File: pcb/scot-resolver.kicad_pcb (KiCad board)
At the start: 2 copper layers, 108.5 x 79.2 mm, 148 parts, among them IC1 AD8692ARMZ, IC10 AD2S1210, IC2 AD8397ARZ, IC3 AD8692ARMZ, IC4 TSR1, IC5 AD8692ARMZ, IC6 AD8692ARMZ, IC7 AD8692ARMZ, IC8 MCP2562, IC9 STM32F0xxKxTx, J1 Conn_01x02_Female, J2 Conn_01x02_Female, J3 Conn_01x02_Female, J4 Conn_01x03_Female, J5 Conn_01x03_Female, J6 Conn_01x03_Female, J7 CONN_01x03, P1 SWD, U1 MCP1703A-5002_SOT223, U2 LT1762, U3 MCP1703A-5002_SOT223, U4 MCP1703A-5002_SOT223, U5 MCP1703A-3302_SOT223, Y1 Crystal_GND24, Y2 Crystal

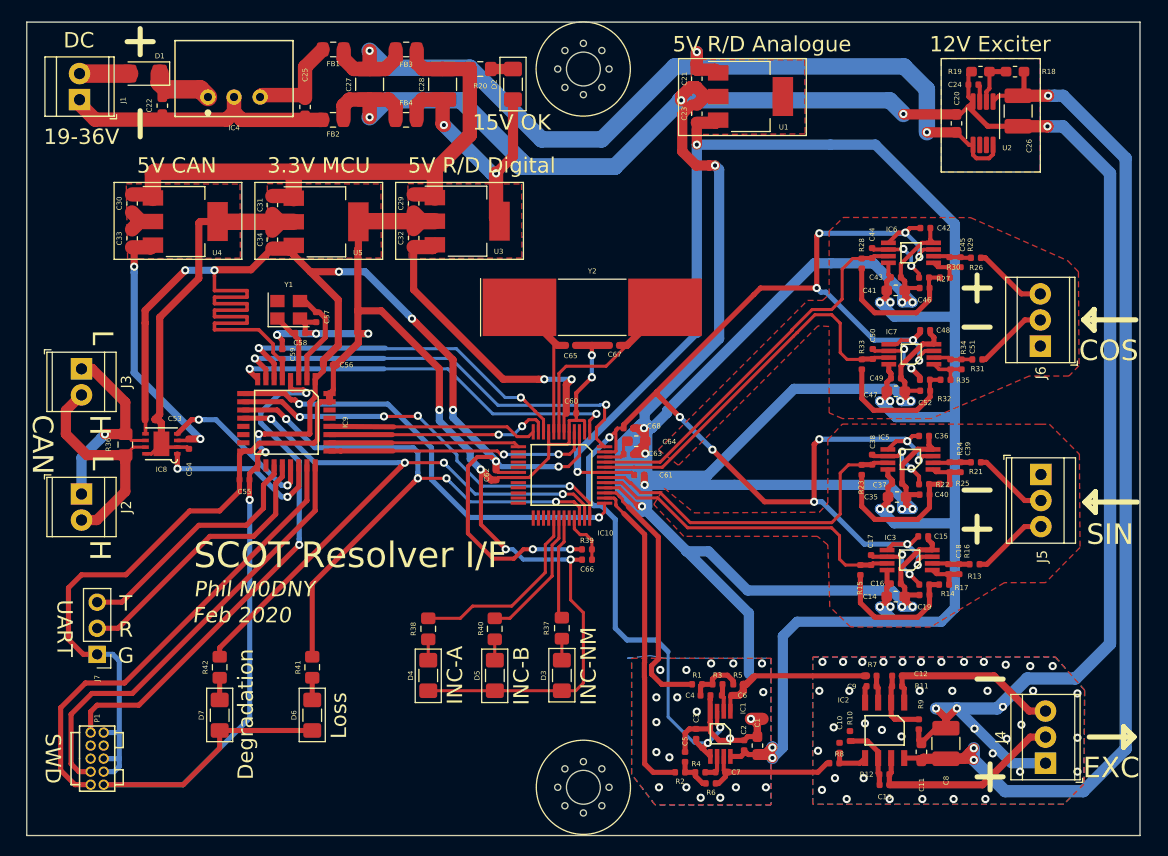
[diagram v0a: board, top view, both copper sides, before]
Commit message: WIP..
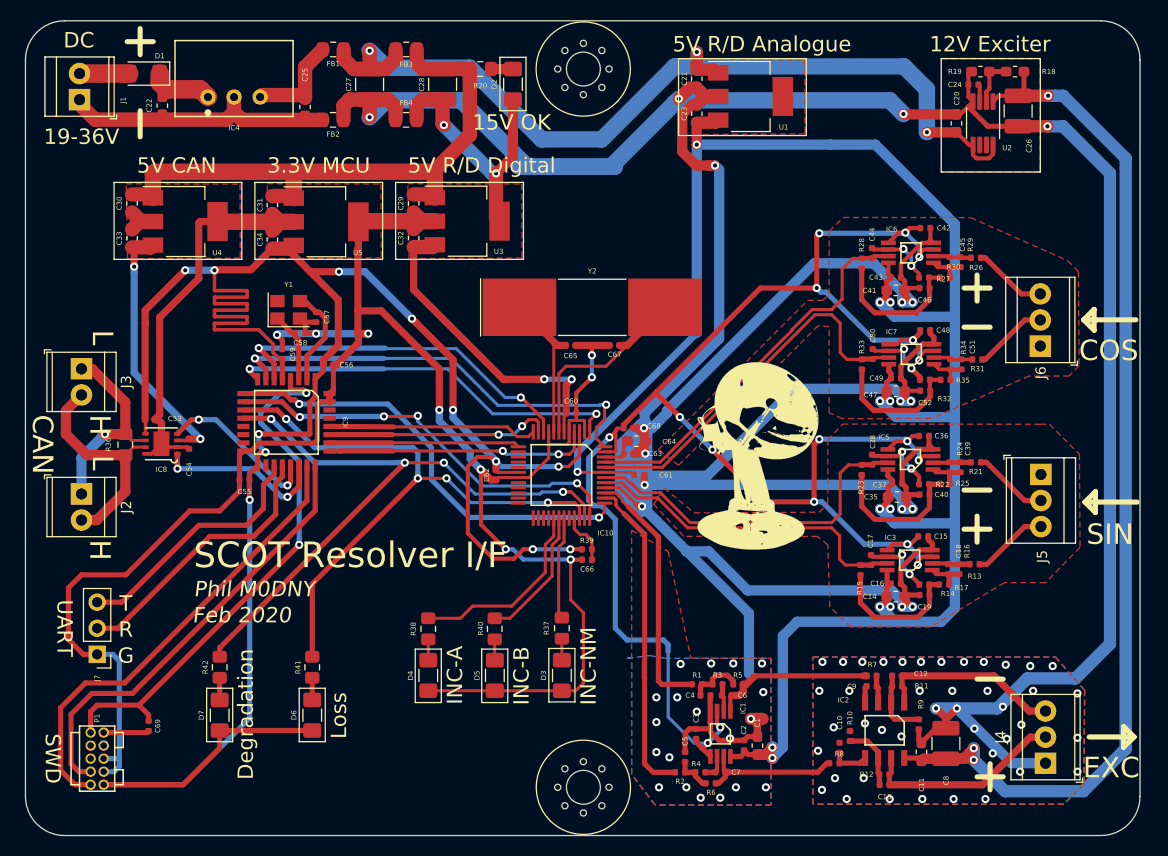
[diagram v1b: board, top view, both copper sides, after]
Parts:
- added C69: 100n, Capacitor_SMD:C_0402_1005Metric, F.Cu at (92.6, 121.4)
- added G***: LOGO, scot_logo:scot_logo, F.Cu at (152.0, 95.1)
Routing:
- net GND: track 278.8 -> 283.3 mm
- net Net-(C69-Pad1): track 51.4 -> 53.3 mm
- net /Microcontroller & Interface/A1: track 39.7 -> 40.4 mm
- net /Resolver Exciter/AD2S1210_EXC-: track 25.1 -> 24.6 mm
- net GNDA: track 480.2 -> 480.6 mm, vias 79 -> 78
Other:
- board size 108.5 x 79.2 mm -> 108.6 x 79.4 mm
- rule trace_min: 0.2 -> 0.15
- rule via_min_size: 0.4 -> 0.3
